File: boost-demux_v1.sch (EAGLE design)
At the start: 33 parts, among them U1 TI_TPS55330, U2 4067D

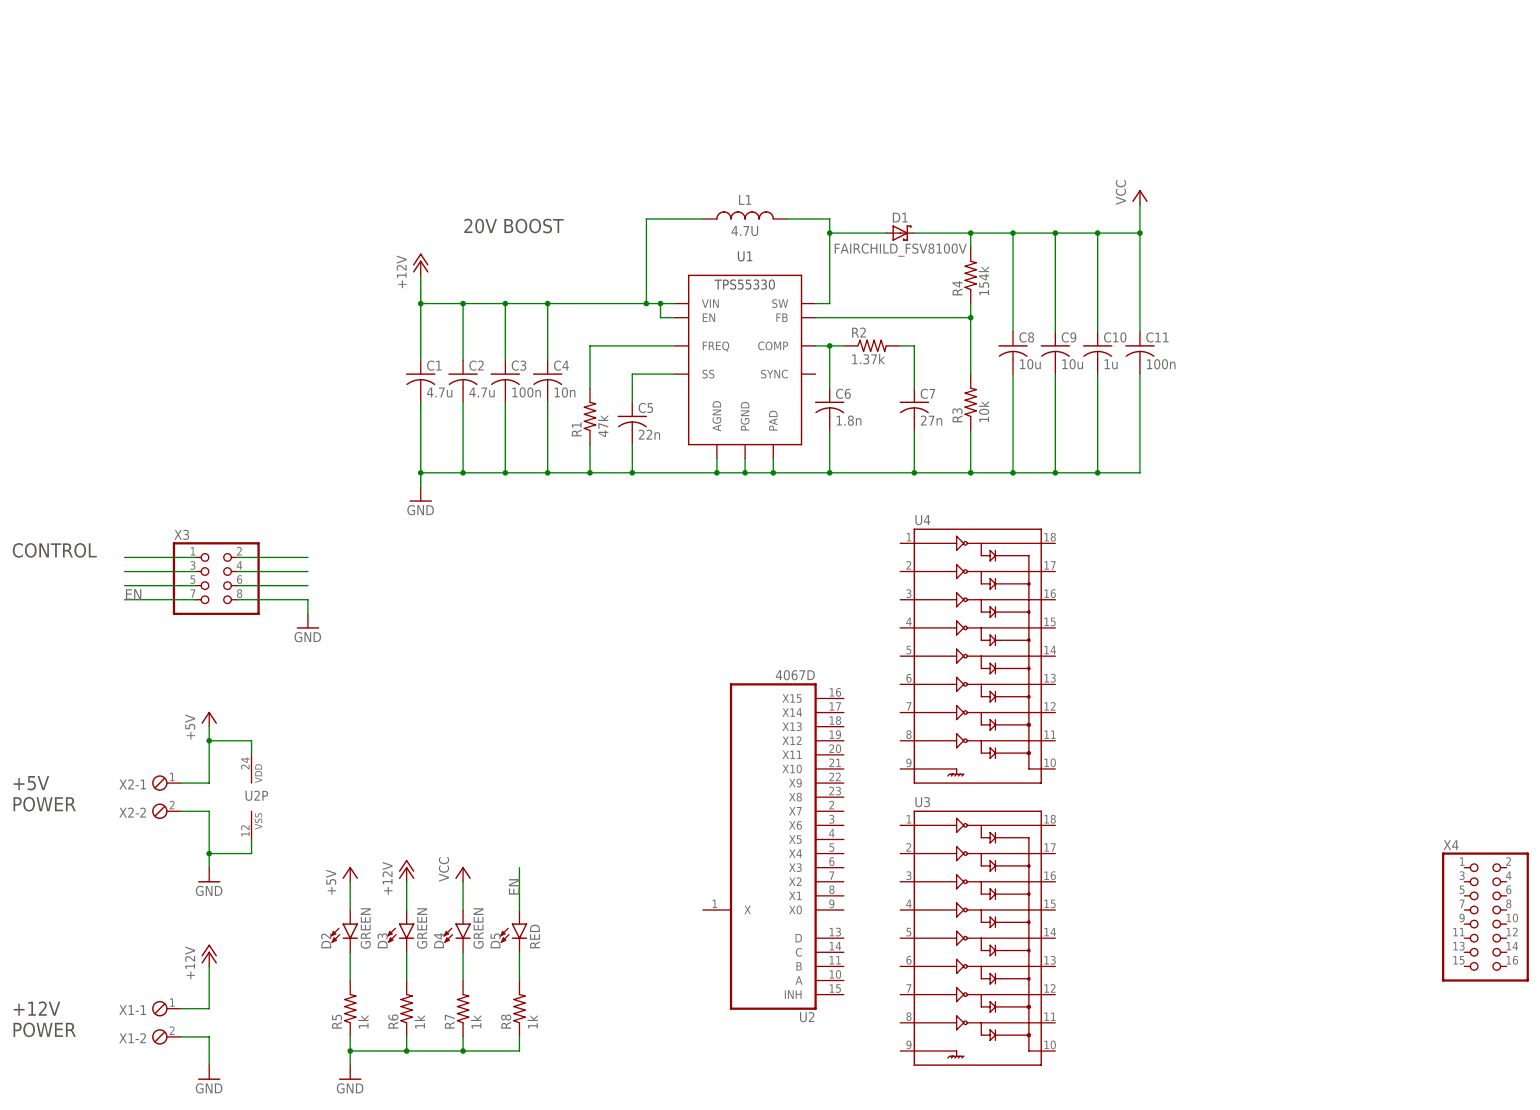
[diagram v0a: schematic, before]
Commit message: PCB draft less markup
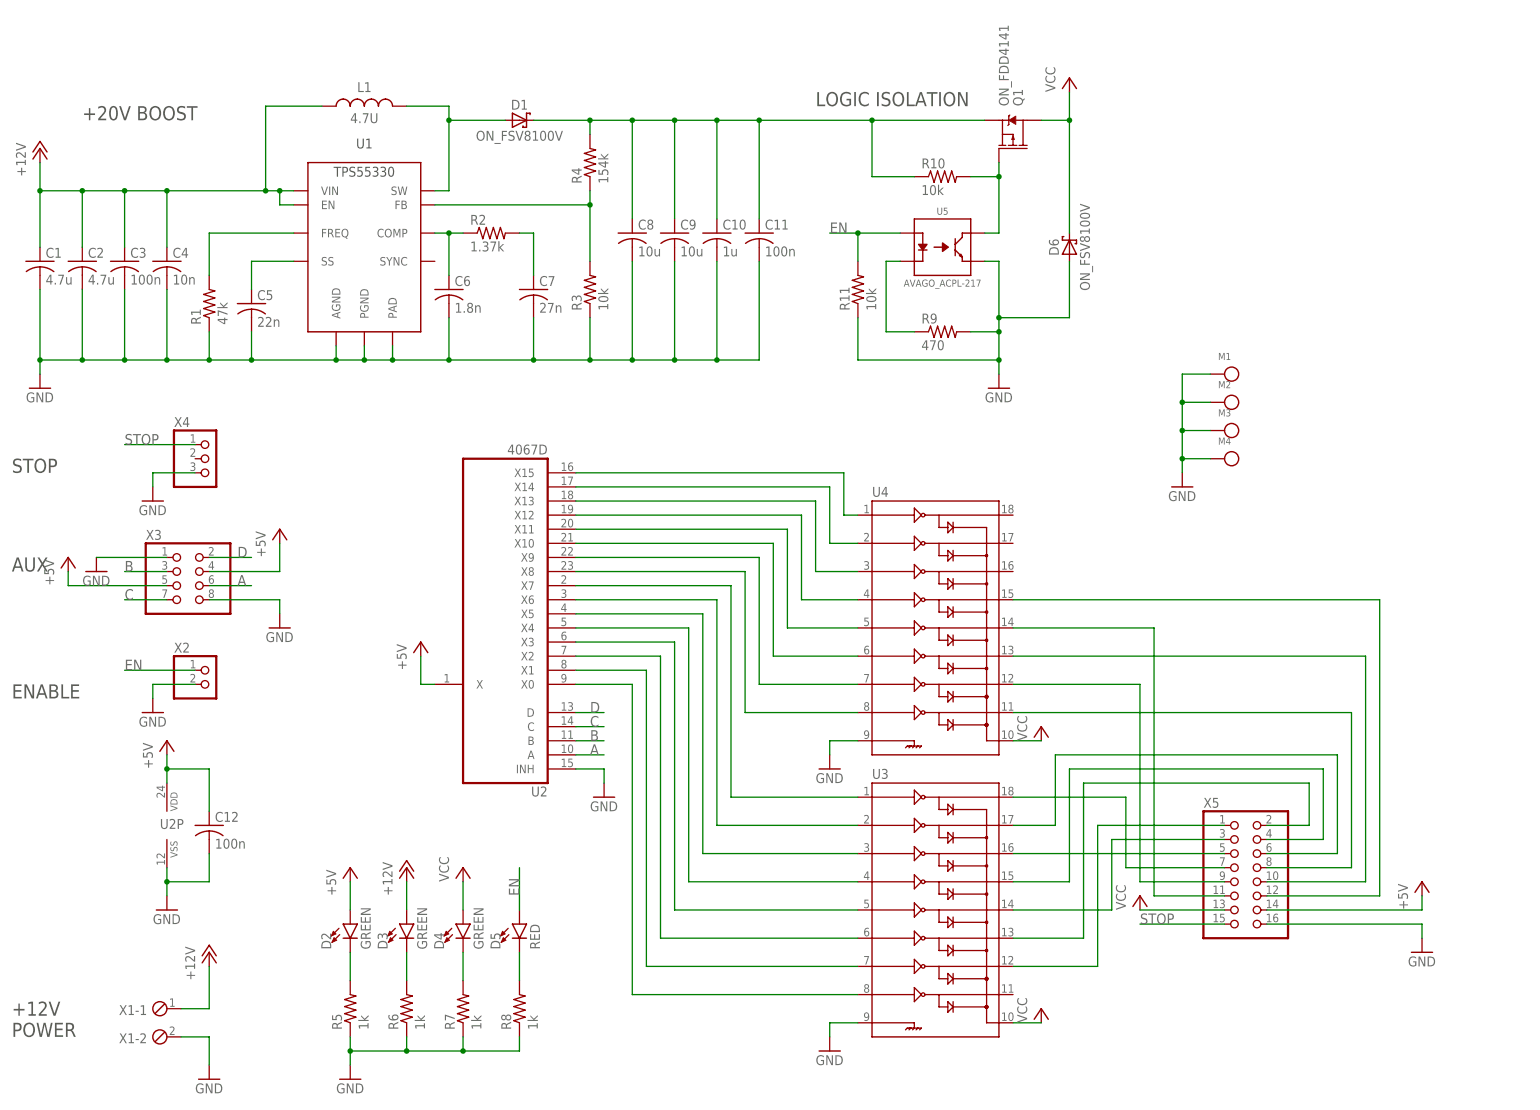
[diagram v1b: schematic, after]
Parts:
- added C12: 100n, rcl:C-USC1206
- added D6: ON_FSV8100V, components:ON_FSV8100V
- added M1, M2, M3, M4: 6-32_MOUNT, components:6-32_MOUNT
- added Q1: ON_FDD4141, components:ON_FDD4141
- added R10, R11: 10k, rcl:R-US_R0805
- added R9: 470, resistor:R-US_R1206
- added U5: AVAGO_ACPL-217, components:AVAGO_ACPL-217
- added X5: (no value), pinhead:PINHD-2X8
- D1: value FAIRCHILD_FSV8100V -> ON_FSV8100V; device components:FAIRCHILD_FSV8100V -> components:ON_FSV8100V
- X2: device con-phoenix-254:MPT2 -> pinhead:PINHD-1X2/90
- X4: device pinhead:PINHD-2X8 -> pinhead:PINHD-1X3/90
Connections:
- new net A: U2A.A, X3.6
- new net B: U2A.B, X3.3
- new net C: U2A.C, X3.7
- new net D: U2A.D, X3.2
- new net N$12: C10.1, C11.1, C8.1, C9.1, D1.C, Q1.S, R10.1, R4.2
- new net N$13: Q1.G, R10.2, U5.P$4
- new net N$19: R9.1, U5.P$2
- new net N$20: U2A.X4, U3.4
- new net N$21: U2A.X5, U3.3
- new net N$22: U2A.X6, U3.2
- new net N$23: U2A.X7, U3.1
- new net N$24: U2A.X8, U4.8
- new net N$25: U2A.X9, U4.7
- new net N$26: U2A.X10, U4.6
- new net N$27: U2A.X11, U4.5
- new net N$28: U2A.X12, U4.4
- new net N$29: U2A.X13, U4.3
- new net N$30: U2A.X14, U4.2
- new net N$31: U2A.X15, U4.1
- new net N$32: U3.14, X5.3
- new net N$33: U3.15, X5.4
- new net N$34: U3.16, X5.5
- new net N$35: U3.17, X5.6
- new net N$36: U3.18, X5.7
- new net N$37: U4.11, X5.8
- new net N$38: U4.12, X5.9
- new net N$39: U4.13, X5.10
- new net N$40: U4.14, X5.11
- new net N$41: U4.15, X5.12
- new net STOP: X4.1, X5.15
- net +5V: now also C12.1, U2A.X, X3.4, X3.5, X5.14; no longer X2-1.1
- net EN: now also R11.2, U5.P$1, X2.1; no longer X3.7
- net GND: now also C12.2, D6.A, M1.P$1, M2.P$1, M3.P$1, M4.P$1, R11.1, R9.2, U2A.INH, U3.9, U4.9, U5.P$3, X2.2, X3.1, X4.3, X5.16; no longer X2-2.1
- net N$11: now also U2A.X0, U3.8; no longer X3.1
- net N$14: now also U3.12, X5.1; no longer X3.5
- net N$15: now also U2A.X1, U3.7; no longer X3.3
- net N$16: now also U2A.X2, U3.6; no longer X3.2
- net N$17: now also U2A.X3, U3.5; no longer X3.4
- net N$18: now also U3.13, X5.2; no longer X3.6
- net VCC: now also D6.C, Q1.D, U3.10, U4.10, X5.13; no longer C10.1, C11.1, C8.1, C9.1, D1.C, R4.2
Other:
- note added: "+20V BOOST"
- note added: "AUX"
- note added: "ENABLE"
- note added: "LOGIC ISOLATION"
- note added: "STOP"
- note removed: "+5V POWER"
- note removed: "20V BOOST"
- note removed: "CONTROL"
- moved on the sheet: C1, C10, C11, C2, C3, C4, C5, C6, C7, C8, C9, D1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
